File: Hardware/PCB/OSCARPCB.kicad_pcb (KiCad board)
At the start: 2 copper layers, 77.5 x 73 mm, 6 parts, among them J1 PINHD_1x8_Male, J2 PINHD_1x8_Male, J4 Servo OUT, J5 Power Input, J6 PINHD_1x2_Female, U2 ESP32-DevKitC

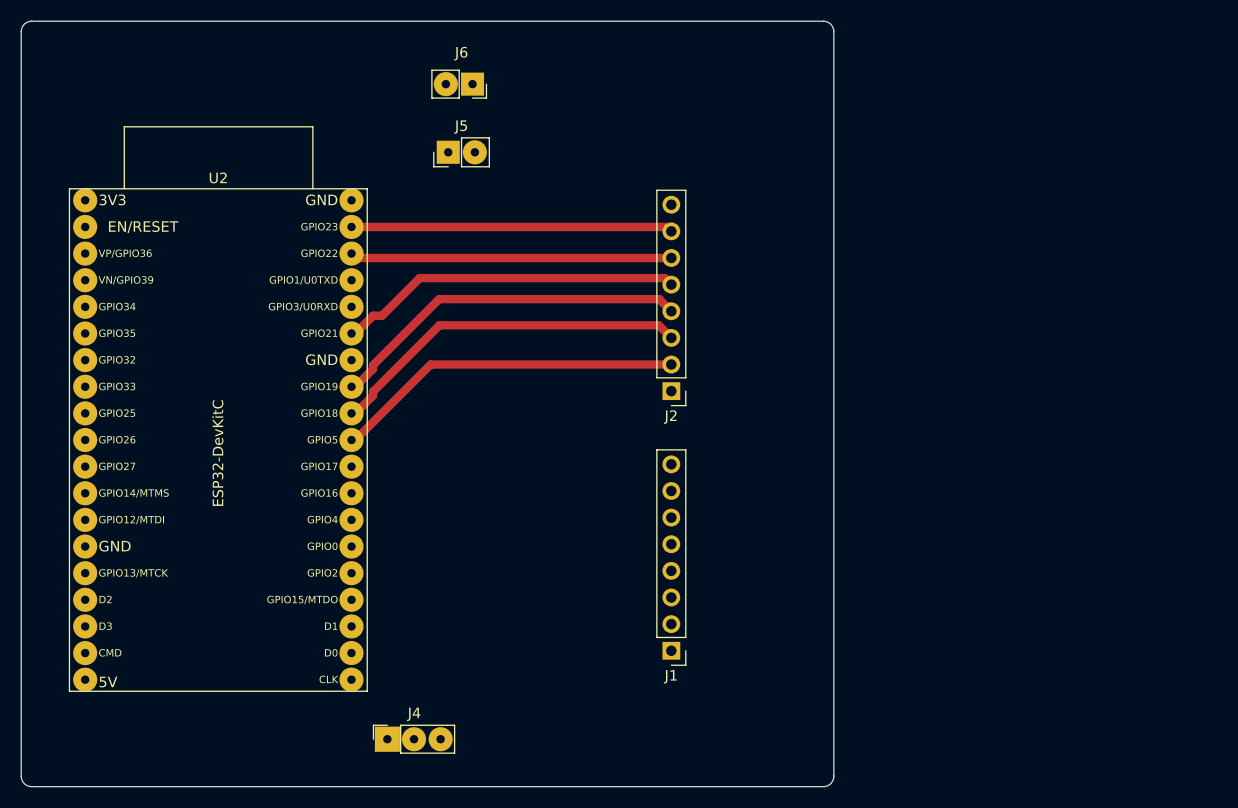
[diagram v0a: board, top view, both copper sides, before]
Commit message: PCB Done?
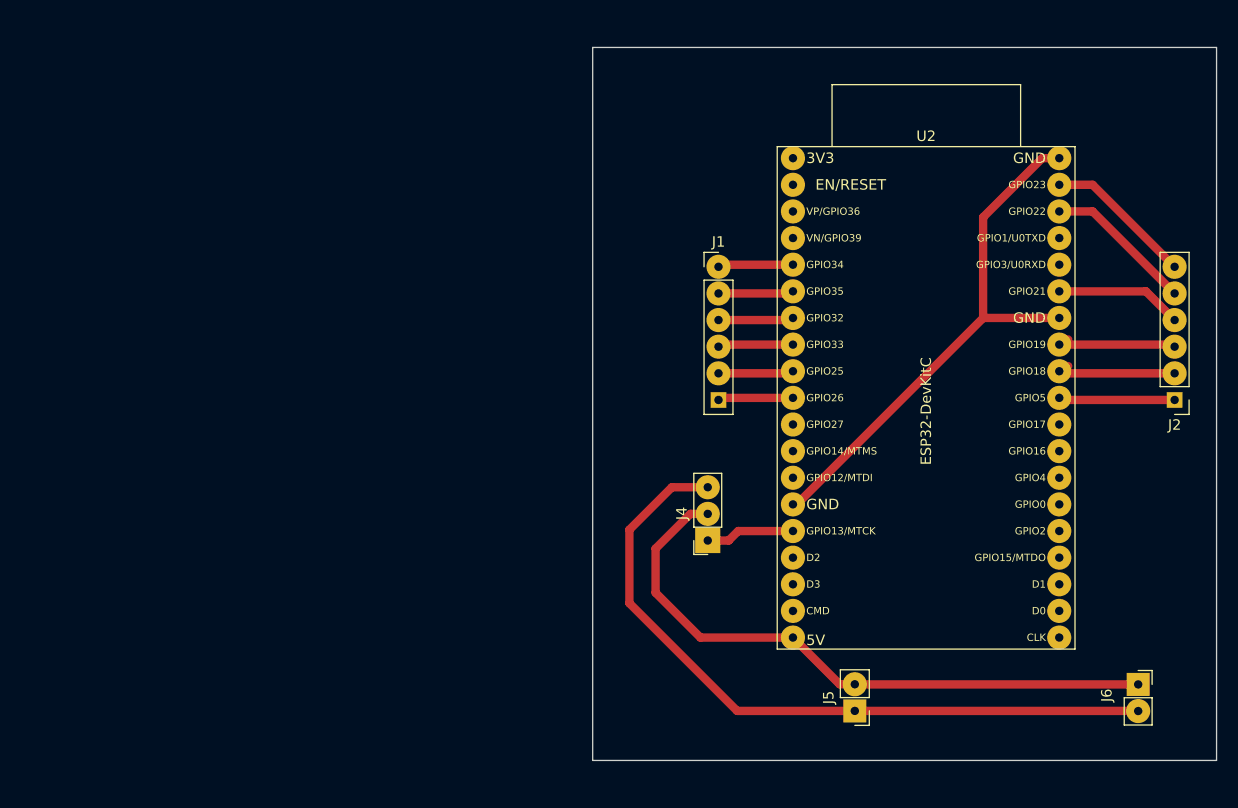
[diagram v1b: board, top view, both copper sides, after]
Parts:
- J1: value PINHD_1x8_Male -> DC Motor; footprint Connector_PinHeader_2.54mm:PinHeader_1x08_P2.54mm_Vertical -> Connector_PinHeader_2.54mm:PinHeader_1x06_P2.54mm_Vertical
- J2: value PINHD_1x8_Male -> Stepper Motor; footprint Connector_PinHeader_2.54mm:PinHeader_1x08_P2.54mm_Vertical -> Connector_PinHeader_2.54mm:PinHeader_1x06_P2.54mm_Vertical
- moved J6 85.5 mm to (136.0, 135.8), turned to 0 degrees
- moved U2 67.6 mm to (103.1, 85.6)
- moved J5 65.9 mm to (109.0, 138.3), turned to 180 degrees
- moved J2 48.0 mm to (139.5, 108.6)
- moved J1 36.9 mm to (96.0, 95.9), turned to 0 degrees
- moved J4 36.0 mm to (95.0, 122.0), turned to 180 degrees
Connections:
- J1 pad 1: VBATT -> L Motor EN
- J1 pad 2: Net-(U2-SD_CLK/GPIO6) -> L Motor 1
- J1 pad 3: Net-(U2-SD_DATA0/GPIO7) -> L Motor 2
- J1 pad 4: Net-(U2-SD_DATA1/GPIO8) -> R Motor 3
- J1 pad 5: R Motor 3 -> R Motor 4
- J1 pad 6: R Motor 4 -> R EN
- J2 pad 1: unconnected-(J2-Pad1) -> Net-(U2-GPIO5)
- J2 pad 2: Net-(U2-GPIO5) -> Net-(U2-GPIO18)
- J2 pad 3: Net-(U2-GPIO18) -> Net-(U2-GPIO19)
- J2 pad 4: Net-(U2-GPIO19) -> Net-(U2-GPIO21)
- J2 pad 5: Net-(U2-GPIO21) -> Net-(U2-GPIO22)
- J2 pad 6: Net-(U2-GPIO22) -> Net-(U2-GPIO23)
- U2 pad 10: unconnected-(U2-DAC_2/ADC2_CH9/GPIO26-Pad10) -> R EN
- U2 pad 20: Net-(U2-SD_CLK/GPIO6) -> unconnected-(U2-SD_CLK/GPIO6-Pad20)
- U2 pad 21: Net-(U2-SD_DATA0/GPIO7) -> unconnected-(U2-SD_DATA0/GPIO7-Pad21)
- U2 pad 22: Net-(U2-SD_DATA1/GPIO8) -> unconnected-(U2-SD_DATA1/GPIO8-Pad22)
- U2 pad 24: R Motor 4 -> unconnected-(U2-ADC2_CH2/GPIO2-Pad24)
- U2 pad 26: R Motor 3 -> unconnected-(U2-ADC2_CH0/GPIO4-Pad26)
- U2 pad 27: R EN -> unconnected-(U2-GPIO16-Pad27)
- U2 pad 28: DIR -> unconnected-(U2-GPIO17-Pad28)
- U2 pad 5: unconnected-(U2-VDET_1/GPIO34/ADC1_CH6-Pad5) -> L Motor EN
- U2 pad 6: unconnected-(U2-VDET_2/GPIO35/ADC1_CH7-Pad6) -> L Motor 1
- U2 pad 7: unconnected-(U2-32K_XP/GPIO32/ADC1_CH4-Pad7) -> L Motor 2
- U2 pad 8: unconnected-(U2-32K_XN/GPIO33/ADC1_CH5-Pad8) -> R Motor 3
- U2 pad 9: unconnected-(U2-DAC_1/ADC2_CH8/GPIO25-Pad9) -> R Motor 4
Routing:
- net GND: track 0.00 -> 120.9 mm
- net VBATT: track 0.00 -> 60.2 mm
- net Net-(U2-GPIO18): track 34.7 -> 12.1 mm
- net Net-(U2-GPIO19): track 34.7 -> 12.1 mm
- net Net-(U2-GPIO5): track 33.5 -> 11.1 mm
- net Net-(U2-GPIO21): track 32.9 -> 12.8 mm
- net Net-(U2-GPIO23): track 30.7 -> 14.2 mm
- net Net-(U2-GPIO22): track 30.7 -> 14.8 mm
- net Net-(U2-MTCK/GPIO13/ADC2_CH4): track 0.00 -> 8.56 mm
- net R Motor 4: track 0.00 -> 7.49 mm
- net L Motor 2: track 0.00 -> 7.49 mm
- net R Motor 3: track 0.00 -> 7.49 mm
- net R EN: track 0.00 -> 7.49 mm
- net L Motor EN: track 0.00 -> 7.49 mm
- net L Motor 1: track 0.00 -> 7.49 mm
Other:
- board size 77.5 x 73 mm -> 59.5 x 68 mm
